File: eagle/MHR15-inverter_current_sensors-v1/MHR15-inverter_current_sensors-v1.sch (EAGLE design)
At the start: 7 parts

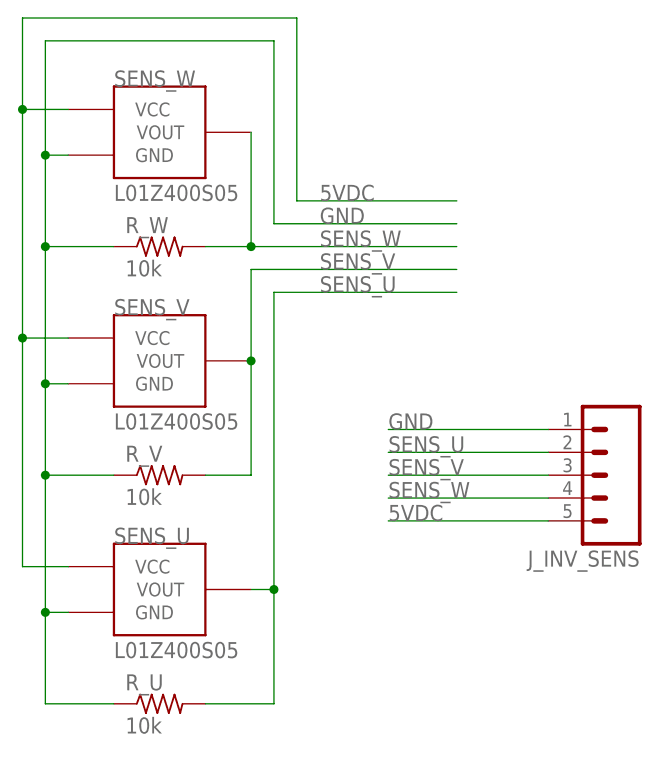
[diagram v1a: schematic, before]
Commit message: updated board, but this version violates clearance
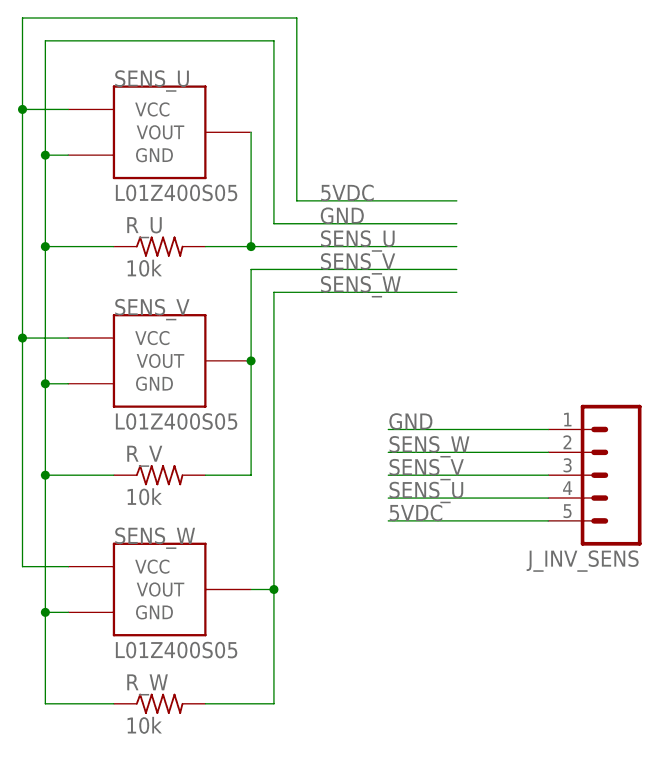
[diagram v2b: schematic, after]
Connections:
- net SENS_U: now also J_INV_SENS.4; no longer J_INV_SENS.2
- net SENS_W: now also J_INV_SENS.2; no longer J_INV_SENS.4
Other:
- moved on the sheet: R_U, R_W, SENS_U, SENS_W
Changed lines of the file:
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@@
 </classes>
 <parts>
+<part name="SENS_U" library="MHR15-TS" deviceset="L01Z400S05" device=""/>
+<part name="SENS_V" library="MHR15-TS" deviceset="L01Z400S05" device=""/>
 <part name="SENS_W" library="MHR15-TS" deviceset="L01Z400S05" device=""/>
-<part name="SENS_V" library="MHR15-TS" deviceset="L01Z400S05" device=""/>
-<part name="SENS_U" library="MHR15-TS" deviceset="L01Z400S05" device=""/>
+<part name="R_U" library="rcl" deviceset="R-US_" device="R0603" value="10k"/>
+<part name="R_V" library="rcl" deviceset="R-US_" device="R0603" value="10k"/>
 <part name="R_W" library="rcl" deviceset="R-US_" device="R0603" value="10k"/>
-<part name="R_V" library="rcl" deviceset="R-US_" device="R0603" value="10k"/>
-<part name="R_U" library="rcl" deviceset="R-US_" device="R0603" value="10k"/>
 <part name="J_INV_SENS" library="SparkFun-Connectors" deviceset="M05" device="LOCK"/>
 </parts>
@@
 </plain>
 <instances>
-<instance part="SENS_W" gate="G$1" x="15.24" y="33.02"/>
+<instance part="SENS_U" gate="G$1" x="15.24" y="33.02"/>
 <instance part="SENS_V" gate="G$1" x="15.24" y="7.62"/>
-<instance part="SENS_U" gate="G$1" x="15.24" y="-17.78"/>
-<instance part="R_W" gate="G$1" x="20.32" y="25.4"/>
+<instance part="SENS_W" gate="G$1" x="15.24" y="-17.78"/>
+<instance part="R_U" gate="G$1" x="20.32" y="25.4"/>
 <instance part="R_V" gate="G$1" x="20.32" y="0"/>
-<instance part="R_U" gate="G$1" x="20.32" y="-25.4"/>
+<instance part="R_W" gate="G$1" x="20.32" y="-25.4"/>
 <instance part="J_INV_SENS" gate="G$1" x="71.12" y="0" rot="R180"/>
 </instances>
@@
 <net name="SENS_W" class="0">
 <segment>
-<pinref part="SENS_W" gate="G$1" pin="VOUT"/>
-<wire x1="53.34" y1="25.4" x2="30.48" y2="25.4" width="0.1524" layer="91"/>
-<wire x1="30.48" y1="25.4" x2="30.48" y2="38.1" width="0.1524" layer="91"/>
-<label x="38.1" y="25.4" size="1.778" layer="95"/>
-<pinref part="R_W" gate="G$1" pin="2"/>
-<wire x1="30.48" y1="25.4" x2="25.4" y2="25.4" width="0.1524" layer="91"/>
-<junction x="30.48" y="25.4"/>
-</segment>
-<segment>
-<pinref part="J_INV_SENS" gate="G$1" pin="4"/>
-<wire x1="45.72" y1="-2.54" x2="63.5" y2="-2.54" width="0.1524" layer="91"/>
-<label x="45.72" y="-2.54" size="1.778" layer="95"/>
-</segment>
-</net>
-<net name="SENS_U" class="0">
-<segment>
 <wire x1="33.02" y1="20.32" x2="53.34" y2="20.32" width="0.1524" layer="91"/>
 <label x="38.1" y="20.32" size="1.778" layer="95"/>
-<pinref part="SENS_U" gate="G$1" pin="VOUT"/>
+<pinref part="SENS_W" gate="G$1" pin="VOUT"/>
 <wire x1="33.02" y1="20.32" x2="33.02" y2="-12.7" width="0.1524" layer="91"/>
 <wire x1="33.02" y1="-12.7" x2="30.48" y2="-12.7" width="0.1524" layer="91"/>
-<pinref part="R_U" gate="G$1" pin="2"/>
+<pinref part="R_W" gate="G$1" pin="2"/>
 <wire x1="33.02" y1="-12.7" x2="33.02" y2="-25.4" width="0.1524" layer="91"/>
 <wire x1="33.02" y1="-25.4" x2="25.4" y2="-25.4" width="0.1524" layer="91"/>
@@
 </segment>
 </net>
+<net name="SENS_U" class="0">
+<segment>
+<pinref part="SENS_U" gate="G$1" pin="VOUT"/>
+<wire x1="53.34" y1="25.4" x2="30.48" y2="25.4" width="0.1524" layer="91"/>
+<wire x1="30.48" y1="25.4" x2="30.48" y2="38.1" width="0.1524" layer="91"/>
+<label x="38.1" y="25.4" size="1.778" layer="95"/>
+<pinref part="R_U" gate="G$1" pin="2"/>
+<wire x1="30.48" y1="25.4" x2="25.4" y2="25.4" width="0.1524" layer="91"/>
+<junction x="30.48" y="25.4"/>
+</segment>
+<segment>
+<pinref part="J_INV_SENS" gate="G$1" pin="4"/>
+<wire x1="45.72" y1="-2.54" x2="63.5" y2="-2.54" width="0.1524" layer="91"/>
+<label x="45.72" y="-2.54" size="1.778" layer="95"/>
+</segment>
+</net>
 <net name="5VDC" class="0">
 <segment>
@@
 <wire x1="35.56" y1="30.48" x2="35.56" y2="50.8" width="0.1524" layer="91"/>
 <wire x1="35.56" y1="50.8" x2="5.08" y2="50.8" width="0.1524" layer="91"/>
-<pinref part="SENS_W" gate="G$1" pin="VCC"/>
+<pinref part="SENS_U" gate="G$1" pin="VCC"/>
 <wire x1="5.08" y1="50.8" x2="5.08" y2="40.64" width="0.1524" layer="91"/>
 <wire x1="5.08" y1="40.64" x2="10.16" y2="40.64" width="0.1524" layer="91"/>
@@
 <wire x1="5.08" y1="40.64" x2="5.08" y2="15.24" width="0.1524" layer="91"/>
 <label x="38.1" y="30.48" size="1.778" layer="95"/>
-<pinref part="SENS_U" gate="G$1" pin="VCC"/>
+<pinref part="SENS_W" gate="G$1" pin="VCC"/>
 <wire x1="5.08" y1="15.24" x2="5.08" y2="-10.16" width="0.1524" layer="91"/>
 <wire x1="10.16" y1="-10.16" x2="5.08" y2="-10.16" width="0.1524" layer="91"/>
@@
 <wire x1="33.02" y1="27.94" x2="53.34" y2="27.94" width="0.1524" layer="91"/>
 <label x="38.1" y="27.94" size="1.778" layer="95"/>
-<pinref part="SENS_W" gate="G$1" pin="GND"/>
+<pinref part="SENS_U" gate="G$1" pin="GND"/>
 <wire x1="7.62" y1="48.26" x2="7.62" y2="35.56" width="0.1524" layer="91"/>
 <wire x1="7.62" y1="35.56" x2="10.16" y2="35.56" width="0.1524" layer="91"/>
-<pinref part="R_W" gate="G$1" pin="1"/>
+<pinref part="R_U" gate="G$1" pin="1"/>
 <wire x1="15.24" y1="25.4" x2="7.62" y2="25.4" width="0.1524" layer="91"/>
 <wire x1="7.62" y1="35.56" x2="7.62" y2="25.4" width="0.1524" layer="91"/>
@@
 <wire x1="7.62" y1="0" x2="15.24" y2="0" width="0.1524" layer="91"/>
 <junction x="7.62" y="10.16"/>
-<pinref part="SENS_U" gate="G$1" pin="GND"/>
+<pinref part="SENS_W" gate="G$1" pin="GND"/>
 <wire x1="7.62" y1="0" x2="7.62" y2="-15.24" width="0.1524" layer="91"/>
 <wire x1="7.62" y1="-15.24" x2="10.16" y2="-15.24" width="0.1524" layer="91"/>
 <junction x="7.62" y="0"/>
-<pinref part="R_U" gate="G$1" pin="1"/>
+<pinref part="R_W" gate="G$1" pin="1"/>
 <wire x1="15.24" y1="-25.4" x2="7.62" y2="-25.4" width="0.1524" layer="91"/>
 <wire x1="7.62" y1="-25.4" x2="7.62" y2="-15.24" width="0.1524" layer="91"/>

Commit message: finalized v1 of current sensor board
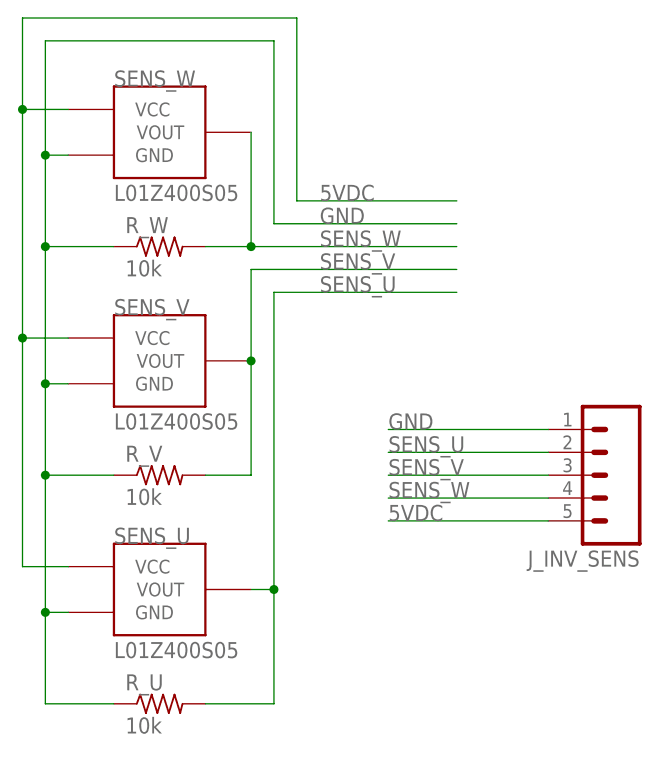
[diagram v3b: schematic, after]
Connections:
- net SENS_U: now also J_INV_SENS.2; no longer J_INV_SENS.4
- net SENS_W: now also J_INV_SENS.4; no longer J_INV_SENS.2
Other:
- moved on the sheet: R_U, R_W, SENS_U, SENS_W
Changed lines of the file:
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@@
 </classes>
 <parts>
+<part name="SENS_W" library="MHR15-TS" deviceset="L01Z400S05" device=""/>
+<part name="SENS_V" library="MHR15-TS" deviceset="L01Z400S05" device=""/>
 <part name="SENS_U" library="MHR15-TS" deviceset="L01Z400S05" device=""/>
-<part name="SENS_V" library="MHR15-TS" deviceset="L01Z400S05" device=""/>
-<part name="SENS_W" library="MHR15-TS" deviceset="L01Z400S05" device=""/>
+<part name="R_W" library="rcl" deviceset="R-US_" device="R0603" value="10k"/>
+<part name="R_V" library="rcl" deviceset="R-US_" device="R0603" value="10k"/>
 <part name="R_U" library="rcl" deviceset="R-US_" device="R0603" value="10k"/>
-<part name="R_V" library="rcl" deviceset="R-US_" device="R0603" value="10k"/>
-<part name="R_W" library="rcl" deviceset="R-US_" device="R0603" value="10k"/>
 <part name="J_INV_SENS" library="SparkFun-Connectors" deviceset="M05" device="LOCK"/>
 </parts>
@@
 </plain>
 <instances>
-<instance part="SENS_U" gate="G$1" x="15.24" y="33.02"/>
+<instance part="SENS_W" gate="G$1" x="15.24" y="33.02"/>
 <instance part="SENS_V" gate="G$1" x="15.24" y="7.62"/>
-<instance part="SENS_W" gate="G$1" x="15.24" y="-17.78"/>
-<instance part="R_U" gate="G$1" x="20.32" y="25.4"/>
+<instance part="SENS_U" gate="G$1" x="15.24" y="-17.78"/>
+<instance part="R_W" gate="G$1" x="20.32" y="25.4"/>
 <instance part="R_V" gate="G$1" x="20.32" y="0"/>
-<instance part="R_W" gate="G$1" x="20.32" y="-25.4"/>
+<instance part="R_U" gate="G$1" x="20.32" y="-25.4"/>
 <instance part="J_INV_SENS" gate="G$1" x="71.12" y="0" rot="R180"/>
 </instances>
@@
 <net name="SENS_W" class="0">
 <segment>
+<pinref part="SENS_W" gate="G$1" pin="VOUT"/>
+<wire x1="53.34" y1="25.4" x2="30.48" y2="25.4" width="0.1524" layer="91"/>
+<wire x1="30.48" y1="25.4" x2="30.48" y2="38.1" width="0.1524" layer="91"/>
+<label x="38.1" y="25.4" size="1.778" layer="95"/>
+<pinref part="R_W" gate="G$1" pin="2"/>
+<wire x1="30.48" y1="25.4" x2="25.4" y2="25.4" width="0.1524" layer="91"/>
+<junction x="30.48" y="25.4"/>
+</segment>
+<segment>
+<pinref part="J_INV_SENS" gate="G$1" pin="4"/>
+<wire x1="45.72" y1="-2.54" x2="63.5" y2="-2.54" width="0.1524" layer="91"/>
+<label x="45.72" y="-2.54" size="1.778" layer="95"/>
+</segment>
+</net>
+<net name="SENS_U" class="0">
+<segment>
 <wire x1="33.02" y1="20.32" x2="53.34" y2="20.32" width="0.1524" layer="91"/>
 <label x="38.1" y="20.32" size="1.778" layer="95"/>
-<pinref part="SENS_W" gate="G$1" pin="VOUT"/>
+<pinref part="SENS_U" gate="G$1" pin="VOUT"/>
 <wire x1="33.02" y1="20.32" x2="33.02" y2="-12.7" width="0.1524" layer="91"/>
 <wire x1="33.02" y1="-12.7" x2="30.48" y2="-12.7" width="0.1524" layer="91"/>
-<pinref part="R_W" gate="G$1" pin="2"/>
+<pinref part="R_U" gate="G$1" pin="2"/>
 <wire x1="33.02" y1="-12.7" x2="33.02" y2="-25.4" width="0.1524" layer="91"/>
 <wire x1="33.02" y1="-25.4" x2="25.4" y2="-25.4" width="0.1524" layer="91"/>
@@
 </segment>
 </net>
-<net name="SENS_U" class="0">
-<segment>
-<pinref part="SENS_U" gate="G$1" pin="VOUT"/>
-<wire x1="53.34" y1="25.4" x2="30.48" y2="25.4" width="0.1524" layer="91"/>
-<wire x1="30.48" y1="25.4" x2="30.48" y2="38.1" width="0.1524" layer="91"/>
-<label x="38.1" y="25.4" size="1.778" layer="95"/>
-<pinref part="R_U" gate="G$1" pin="2"/>
-<wire x1="30.48" y1="25.4" x2="25.4" y2="25.4" width="0.1524" layer="91"/>
-<junction x="30.48" y="25.4"/>
-</segment>
-<segment>
-<pinref part="J_INV_SENS" gate="G$1" pin="4"/>
-<wire x1="45.72" y1="-2.54" x2="63.5" y2="-2.54" width="0.1524" layer="91"/>
-<label x="45.72" y="-2.54" size="1.778" layer="95"/>
-</segment>
-</net>
 <net name="5VDC" class="0">
 <segment>
@@
 <wire x1="35.56" y1="30.48" x2="35.56" y2="50.8" width="0.1524" layer="91"/>
 <wire x1="35.56" y1="50.8" x2="5.08" y2="50.8" width="0.1524" layer="91"/>
-<pinref part="SENS_U" gate="G$1" pin="VCC"/>
+<pinref part="SENS_W" gate="G$1" pin="VCC"/>
 <wire x1="5.08" y1="50.8" x2="5.08" y2="40.64" width="0.1524" layer="91"/>
 <wire x1="5.08" y1="40.64" x2="10.16" y2="40.64" width="0.1524" layer="91"/>
@@
 <wire x1="5.08" y1="40.64" x2="5.08" y2="15.24" width="0.1524" layer="91"/>
 <label x="38.1" y="30.48" size="1.778" layer="95"/>
-<pinref part="SENS_W" gate="G$1" pin="VCC"/>
+<pinref part="SENS_U" gate="G$1" pin="VCC"/>
 <wire x1="5.08" y1="15.24" x2="5.08" y2="-10.16" width="0.1524" layer="91"/>
 <wire x1="10.16" y1="-10.16" x2="5.08" y2="-10.16" width="0.1524" layer="91"/>
@@
 <wire x1="33.02" y1="27.94" x2="53.34" y2="27.94" width="0.1524" layer="91"/>
 <label x="38.1" y="27.94" size="1.778" layer="95"/>
-<pinref part="SENS_U" gate="G$1" pin="GND"/>
+<pinref part="SENS_W" gate="G$1" pin="GND"/>
 <wire x1="7.62" y1="48.26" x2="7.62" y2="35.56" width="0.1524" layer="91"/>
 <wire x1="7.62" y1="35.56" x2="10.16" y2="35.56" width="0.1524" layer="91"/>
-<pinref part="R_U" gate="G$1" pin="1"/>
+<pinref part="R_W" gate="G$1" pin="1"/>
 <wire x1="15.24" y1="25.4" x2="7.62" y2="25.4" width="0.1524" layer="91"/>
 <wire x1="7.62" y1="35.56" x2="7.62" y2="25.4" width="0.1524" layer="91"/>
@@
 <wire x1="7.62" y1="0" x2="15.24" y2="0" width="0.1524" layer="91"/>
 <junction x="7.62" y="10.16"/>
-<pinref part="SENS_W" gate="G$1" pin="GND"/>
+<pinref part="SENS_U" gate="G$1" pin="GND"/>
 <wire x1="7.62" y1="0" x2="7.62" y2="-15.24" width="0.1524" layer="91"/>
 <wire x1="7.62" y1="-15.24" x2="10.16" y2="-15.24" width="0.1524" layer="91"/>
 <junction x="7.62" y="0"/>
-<pinref part="R_W" gate="G$1" pin="1"/>
+<pinref part="R_U" gate="G$1" pin="1"/>
 <wire x1="15.24" y1="-25.4" x2="7.62" y2="-25.4" width="0.1524" layer="91"/>
 <wire x1="7.62" y1="-25.4" x2="7.62" y2="-15.24" width="0.1524" layer="91"/>
